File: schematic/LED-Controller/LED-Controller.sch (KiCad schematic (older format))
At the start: 17 parts

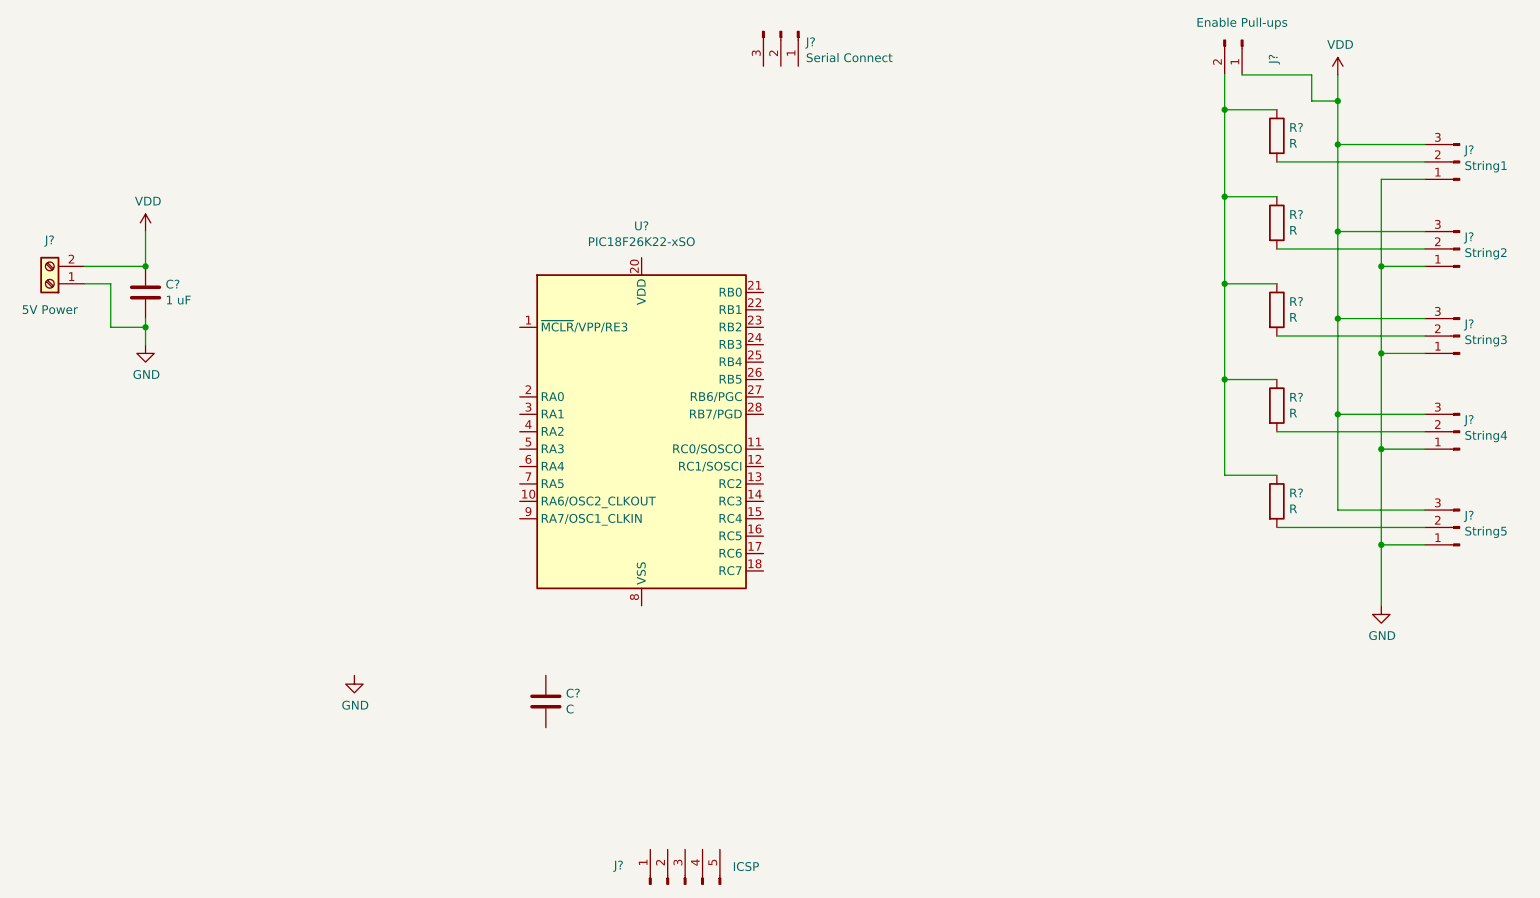
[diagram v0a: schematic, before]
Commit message: Schematic first draft
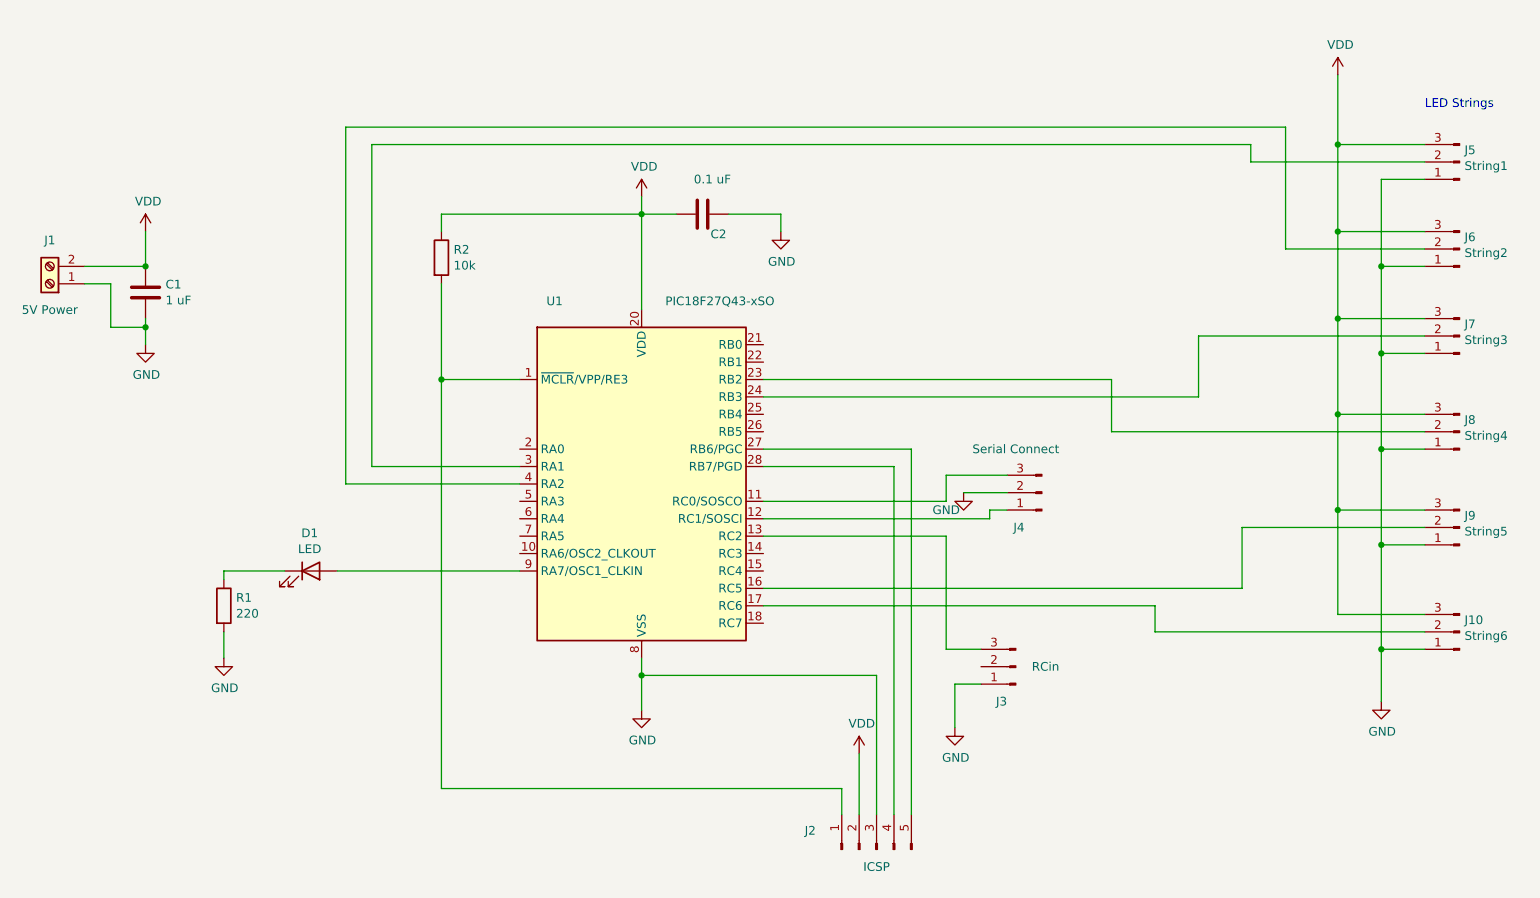
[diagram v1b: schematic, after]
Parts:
- removed J?: Enable Pull-ups, symbol Connector:Conn_01x02_Male
- removed R? (x5): R, symbol Device:R
- added D1: LED, LED_SMD:LED_0603_1608Metric_Pad1.05x0.95mm_HandSolder, symbol Device:LED
- added J10: String6, Connector_Wire:SolderWire-1sqmm_1x03_P7.8mm_D1.4mm_OD3.9mm, symbol Connector:Conn_01x03_Male
- added J3: RCin, Connector_PinHeader_2.54mm:PinHeader_1x03_P2.54mm_Horizontal, symbol Connector:Conn_01x03_Male
- added R1: 220, Resistor_SMD:R_0603_1608Metric, symbol Device:R
- added R2: 10k, Resistor_SMD:R_0603_1608Metric, symbol Device:R
- C1: renamed from C?; footprint (none) -> Capacitor_SMD:C_1206_3216Metric_Pad1.33x1.80mm_HandSolder
- C2: renamed from C?; value C -> 0.1 uF; footprint (none) -> Capacitor_SMD:C_0603_1608Metric_Pad1.08x0.95mm_HandSolder
- J1: renamed from J?; footprint (none) -> Connector_Wire:SolderWire-2.5sqmm_1x02_P8.8mm_D2.4mm_OD4.4mm
- J4: renamed from J?; footprint (none) -> Connector_PinHeader_2.54mm:PinHeader_1x03_P2.54mm_Vertical
- J5, J6, J7, J8, J9: renamed from J?; footprint (none) -> Connector_Wire:SolderWire-1sqmm_1x03_P7.8mm_D1.4mm_OD3.9mm
- U1: renamed from U?; value PIC18F26K22-xSO -> PIC18F27Q43-xSO
- gave numbers to parts that had none: 1
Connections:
- net GND: now also C2.1, J2.3 (Pin_3), J4.2 (Pin_2), U1.19 (VSS), U1.8 (VSS), J10.1 (Pin_1), J3.1 (Pin_1), R1.2
- net VDD: now also C2.2, J2.2 (Pin_2), U1.20 (VDD), J10.3 (Pin_3), R2.1
- net at J4.1 (Pin_1): now also U1.12 (RC1/SOSCI)
- net at J4.3 (Pin_3): now also U1.11 (RC0/SOSCO)
- net at J5.2 (Pin_2): now also U1.3 (RA1)
- net at J6.2 (Pin_2): now also U1.4 (RA2)
- net at J7.2 (Pin_2): now also U1.24 (RB3)
- net at J8.2 (Pin_2): now also U1.23 (RB2)
- net at J9.2 (Pin_2): now also U1.16 (RC5)
- net at U1.1 (~MCLR~/VPP/RE3): now also J2.1 (Pin_1), R2.2
- net at U1.13 (RC2): now also J3.3 (Pin_3)
- net at U1.17 (RC6): now also J10.2 (Pin_2)
- net at U1.27 (RB6/PGC): now also J2.5 (Pin_5)
- net at U1.28 (RB7/PGD): now also J2.4 (Pin_4)
- net at U1.9 (RA7/OSC1_CLKIN): now also D1.2 (A)
- new net: D1.1 (K), R1.1
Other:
- note added: "LED Strings"
- moved on the sheet: C2, J2, J4, U1
